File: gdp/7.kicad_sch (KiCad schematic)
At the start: 8 parts, among them IC1 74LS74, IC15A 74LS367, IC2 74LS42, IC21 74LS374, IC28 74LS374, IC35 74LS374, IC48 74LS374, IC9 74LS374

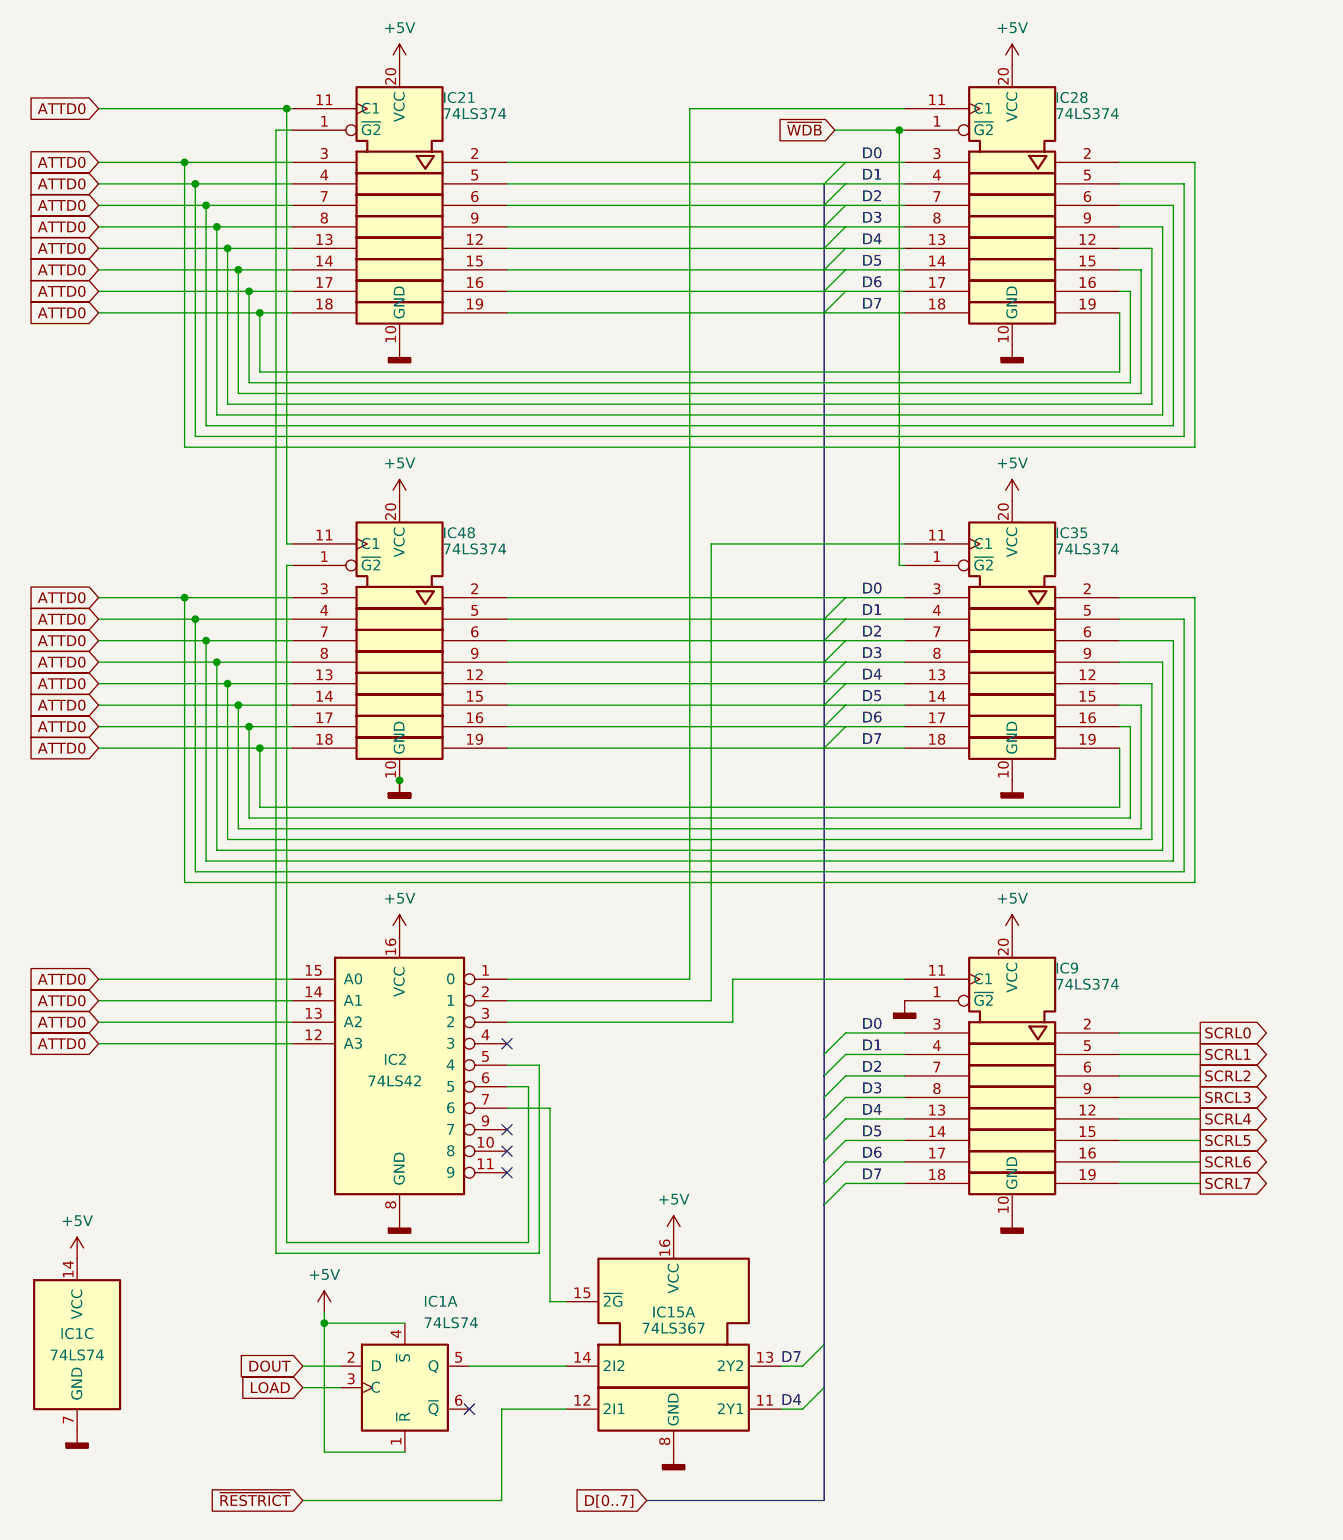
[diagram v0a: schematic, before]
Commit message: Adds Sheet 12
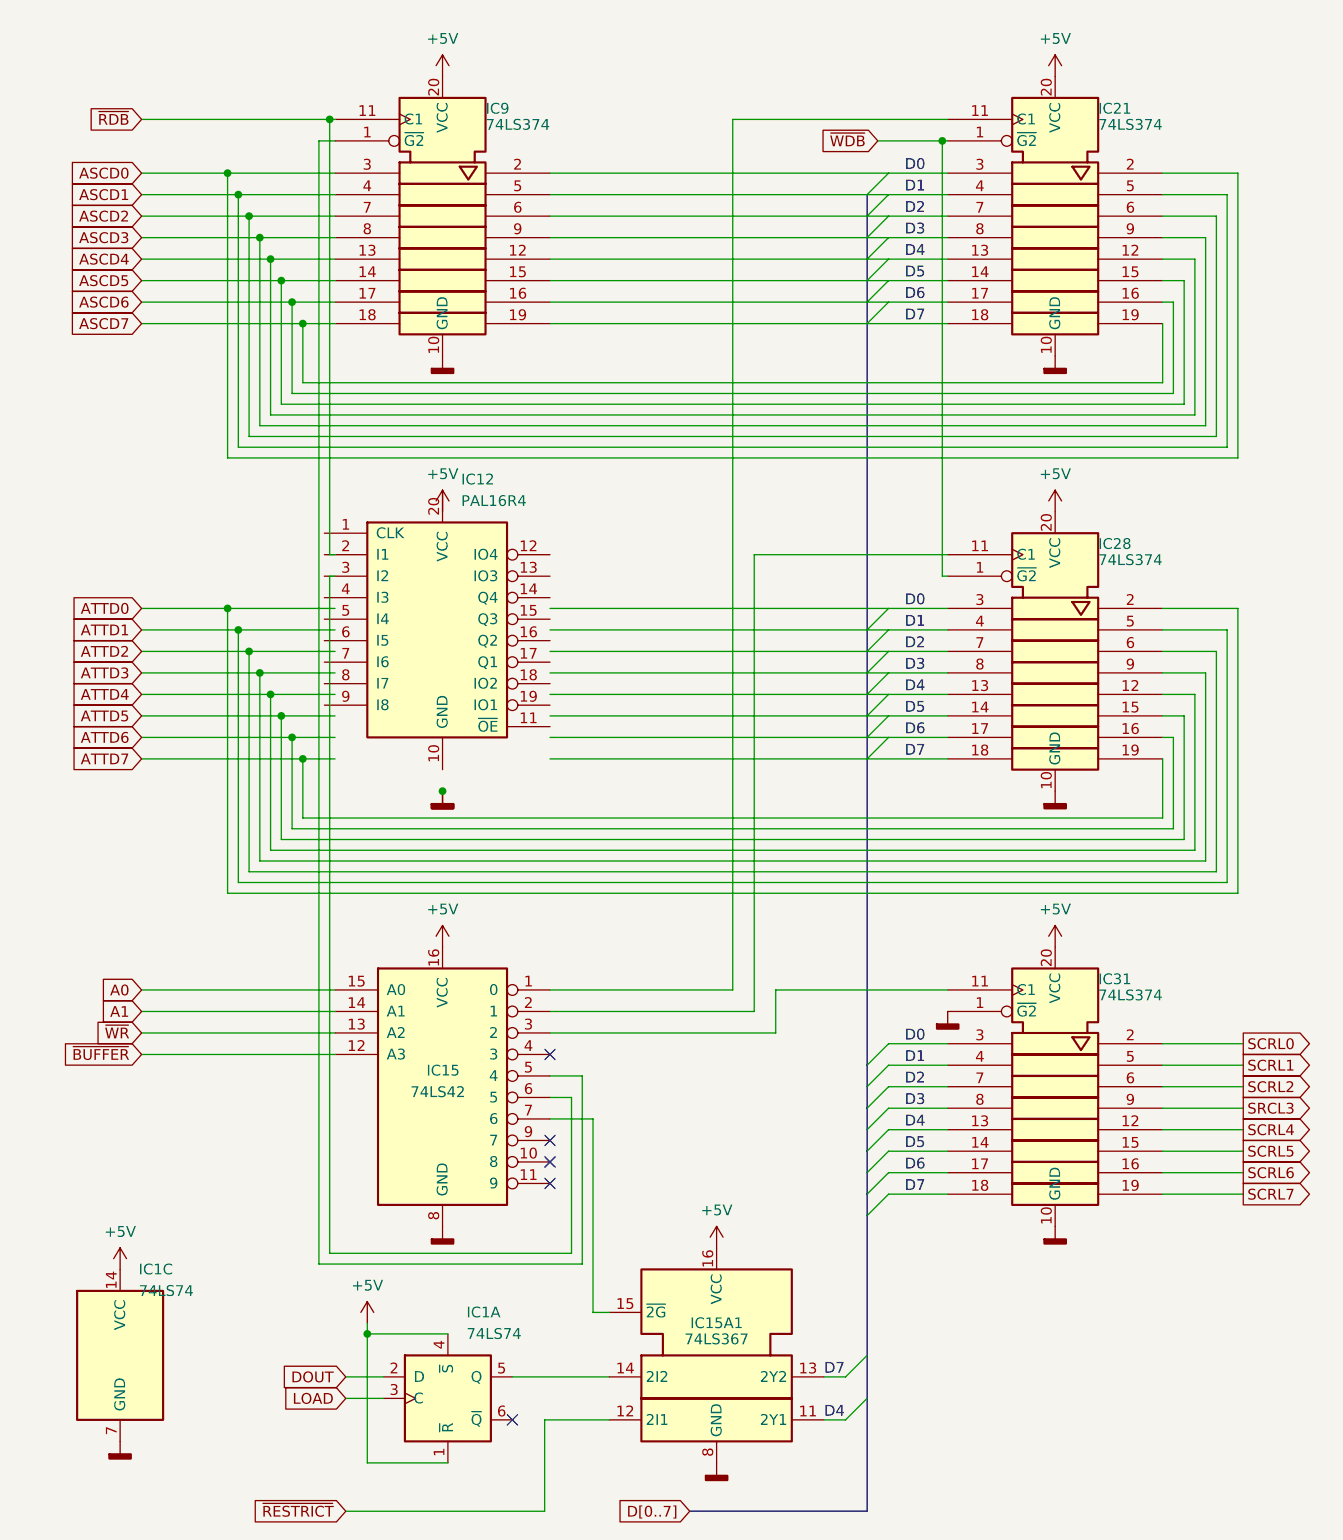
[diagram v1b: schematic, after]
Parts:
- removed IC15A: 74LS367, symbol 74xx_IEEE:74LS367
- removed IC2: 74LS42, symbol 74xx:74LS42
- removed IC35, IC48: 74LS374, symbol 4xxx_IEEE:40374
- added IC12: PAL16R4, symbol 4xxx_IEEE:40374
- added IC15: 74LS42, symbol 74xx:74LS42
- added IC15A1: 74LS367, symbol 74xx_IEEE:74LS367
- added IC31: 74LS374, symbol 4xxx_IEEE:40374
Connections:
- net +5V: now also IC15.16 (VCC), IC15A1.16 (VCC), IC31.20 (VCC)
- net ATTD0: no longer IC21.11 (C1), IC21.13, IC21.14, IC21.17, IC21.18, IC21.3, IC21.4, IC21.7, IC21.8, IC28.12, IC28.15, IC28.16, IC28.19, IC28.5, IC28.6, IC28.9
- net D0: now also IC21.3, IC9.2, IC31.3; no longer IC21.2, IC9.3
- net D1: now also IC21.4, IC9.5, IC31.4; no longer IC21.5, IC9.4
- net D2: now also IC21.7, IC9.6, IC31.7; no longer IC21.6, IC9.7
- net D3: now also IC21.8, IC9.9, IC31.8; no longer IC21.9, IC9.8
- net D4: now also IC21.13, IC9.12, IC15A1.11 (2Y1), IC31.13; no longer IC21.12, IC9.13
- net D5: now also IC21.14, IC9.15, IC31.14; no longer IC21.15, IC9.14
- net D6: now also IC21.17, IC9.16, IC31.17; no longer IC21.16, IC9.17
- net D7: now also IC21.18, IC9.19, IC15A1.13 (2Y2), IC31.18; no longer IC21.19, IC9.18
- net GNDD: now also IC15.8 (GND), IC15A1.8 (GND), IC31.1 (~{G2}), IC31.10 (GND); no longer IC9.1 (~{G2})
- net SCRL0: now also IC31.2; no longer IC9.2
- net SCRL1: now also IC31.5; no longer IC9.5
- net SCRL2: now also IC31.6; no longer IC9.6
- net SCRL4: now also IC31.12; no longer IC9.12
- net SCRL5: now also IC31.15; no longer IC9.15
- net SCRL6: now also IC31.16; no longer IC9.16
- net SCRL7: now also IC31.19; no longer IC9.19
- net SRCL3: now also IC31.9; no longer IC9.9
- net ~{RESTRICT}: now also IC15A1.12 (2I1)
- net ~{WDB}: now also IC21.1 (~{G2})
- net ~{RDB}: now reaches IC9.11 (C1)
- net at IC1.5 (Q): now also IC15A1.14 (2I2)
- net at IC28.11 (C1): now also IC15.2 (1)
- new net: IC15.3 (2), IC31.11 (C1)
- new net: IC15.1 (0), IC21.11 (C1)
- new net: IC15.5 (4), IC9.1 (~{G2})
- new net: IC15.7 (6), IC15A1.15 (~{2G})
- new net A0: IC15.15 (A0)
- new net A1: IC15.14 (A1)
- new net ASCD0: IC21.2, IC9.3
- new net ASCD1: IC21.5, IC9.4
- new net ASCD2: IC21.6, IC9.7
- new net ASCD3: IC21.9, IC9.8
- new net ASCD4: IC21.12, IC9.13
- new net ASCD5: IC21.15, IC9.14
- new net ASCD6: IC21.16, IC9.17
- new net ASCD7: IC21.19, IC9.18
- new net ATTD1: IC28.5
- new net ATTD2: IC28.6
- new net ATTD3: IC28.9
- new net ATTD4: IC28.12
- new net ATTD5: IC28.15
- new net ATTD6: IC28.16
- new net ATTD7: IC28.19
- new net ~{BUFFER}: IC15.12 (A3)
- new net ~{WR}: IC15.13 (A2)

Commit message: Fixes Sheet 7
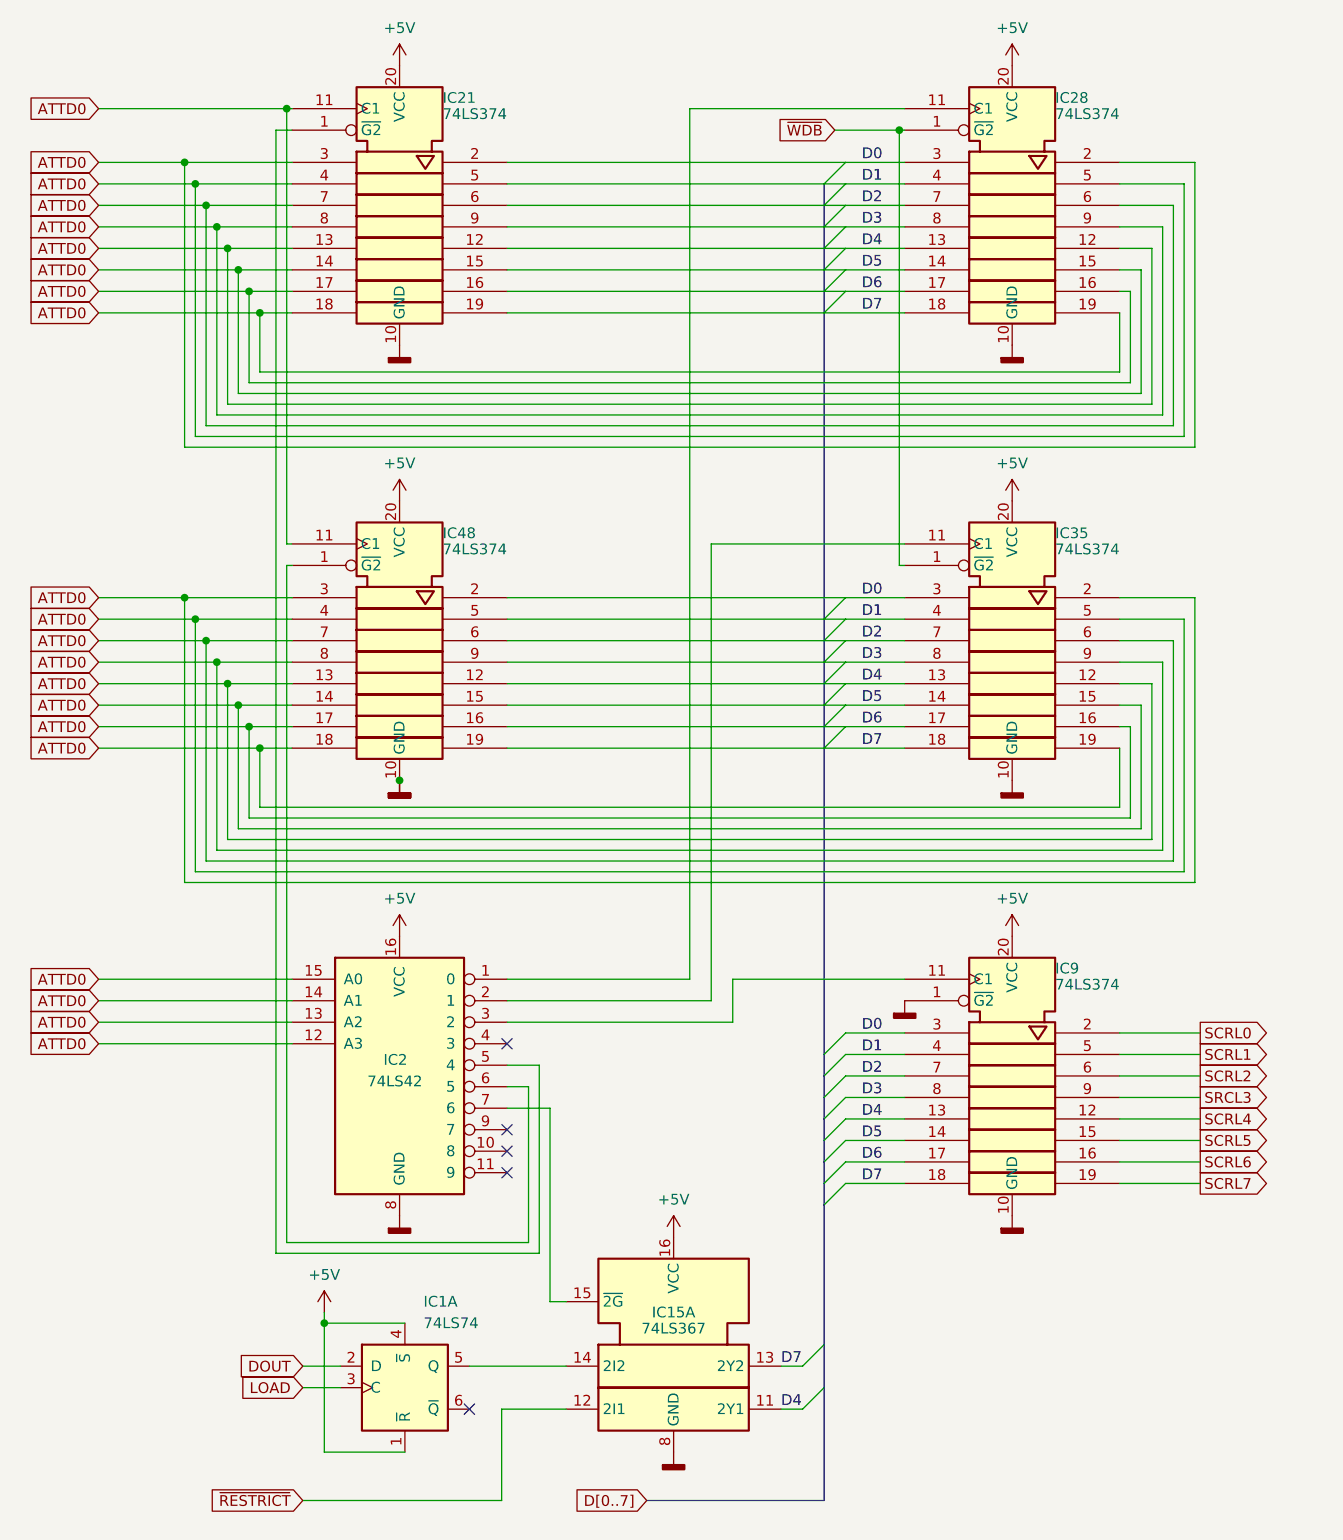
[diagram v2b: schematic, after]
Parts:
- removed unit 3 of IC1
- removed IC12: PAL16R4, symbol 4xxx_IEEE:40374
- removed IC15: 74LS42, symbol 74xx:74LS42
- removed IC15A1: 74LS367, symbol 74xx_IEEE:74LS367
- removed IC31: 74LS374, symbol 4xxx_IEEE:40374
- added IC15A: 74LS367, symbol 74xx_IEEE:74LS367
- added IC2: 74LS42, symbol 74xx:74LS42
- added IC35, IC48: 74LS374, symbol 4xxx_IEEE:40374
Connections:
- net ASCD0 is gone; now on net D0: IC21.2, IC9.3
- net ASCD1 is gone; now on net D1: IC21.5, IC9.4
- net ASCD2 is gone; now on net D2: IC21.6, IC9.7
- net ASCD3 is gone; now on net D3: IC21.9, IC9.8
- net ASCD4 is gone; now on net D4: IC21.12, IC9.13
- net ASCD5 is gone; now on net D5: IC21.15, IC9.14
- net ASCD6 is gone; now on net D6: IC21.16, IC9.17
- net ASCD7 is gone; now on net D7: IC21.19, IC9.18
- net ATTD1 is gone; now on net ATTD0: IC28.5
- net ATTD2 is gone; now on net ATTD0: IC28.6
- net ATTD3 is gone; now on net ATTD0: IC28.9
- net ATTD4 is gone; now on net ATTD0: IC28.12
- net ATTD5 is gone; now on net ATTD0: IC28.15
- net ATTD6 is gone; now on net ATTD0: IC28.16
- net ATTD7 is gone; now on net ATTD0: IC28.19
- net +5V: now also IC15A.16 (VCC), IC2.16 (VCC), IC35.20 (VCC), IC48.20 (VCC)
- net ATTD0: now also IC21.11 (C1), IC21.13, IC21.14, IC21.17, IC21.18, IC21.3, IC21.4, IC21.7, IC21.8, IC2.12 (A3), IC2.13 (A2), IC2.14 (A1), IC2.15 (A0), IC35.12, IC35.15, IC35.16, IC35.19, IC35.2, IC35.5, IC35.6, IC35.9, IC48.11 (C1), IC48.13, IC48.14, IC48.17, IC48.18, IC48.3, IC48.4, IC48.7, IC48.8
- net D0: now also IC35.3, IC48.2; no longer IC21.3, IC9.2
- net D1: now also IC35.4, IC48.5; no longer IC21.4, IC9.5
- net D2: now also IC35.7, IC48.6; no longer IC21.7, IC9.6
- net D3: now also IC35.8, IC48.9; no longer IC21.8, IC9.9
- net D4: now also IC15A.11 (2Y1), IC35.13, IC48.12; no longer IC21.13, IC9.12
- net D5: now also IC35.14, IC48.15; no longer IC21.14, IC9.15
- net D6: now also IC35.17, IC48.16; no longer IC21.17, IC9.16
- net D7: now also IC15A.13 (2Y2), IC35.18, IC48.19; no longer IC21.18, IC9.19
- net GNDD: now also IC9.1 (~{G2}), IC15A.8 (GND), IC2.8 (GND), IC35.10 (GND), IC48.10 (GND)
- net SCRL0: now also IC9.2
- net SCRL1: now also IC9.5
- net SCRL2: now also IC9.6
- net SCRL4: now also IC9.12
- net SCRL5: now also IC9.15
- net SCRL6: now also IC9.16
- net SCRL7: now also IC9.19
- net SRCL3: now also IC9.9
- net ~{RESTRICT}: now also IC15A.12 (2I1)
- net ~{WDB}: now also IC35.1 (~{G2}); no longer IC21.1 (~{G2})
- net at IC1.5 (Q): now also IC15A.14 (2I2)
- net at IC28.11 (C1): now also IC2.1 (0)
- net ~{RDB}: no longer names the net of IC9.11 (C1)
- net ~{RDB}: now also IC2.3 (2)
- new net: IC2.5 (4), IC21.1 (~{G2})
- new net: IC2.2 (1), IC35.11 (C1)
- new net: IC2.6 (5), IC48.1 (~{G2})
- new net: IC15A.15 (~{2G}), IC2.7 (6)
